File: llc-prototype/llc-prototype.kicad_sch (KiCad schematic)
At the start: 37 parts, among them J1 +HV, J2 -HV, J3 +LV, J4 -LV, Q1 MCTL011N20YH-TP, Q2 MCTL011N20YH-TP, Q3 NTMFS1D3N04XMT1G, Q4 NTMFS1D3N04XMT1G, T1 Transformer_SP_2S, U3 PC817, U4 TL431DBZ

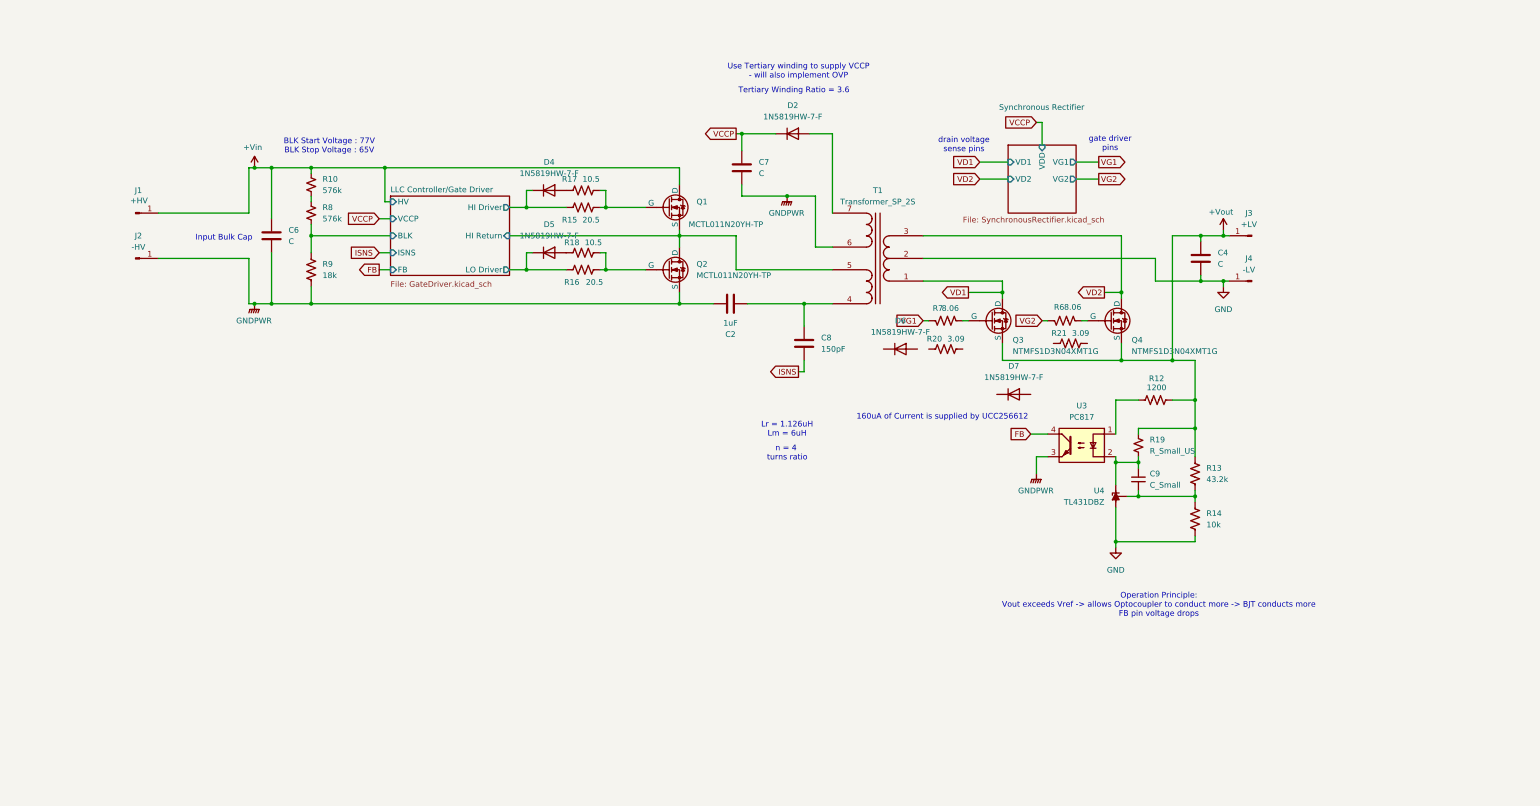
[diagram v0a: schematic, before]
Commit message: added fuses
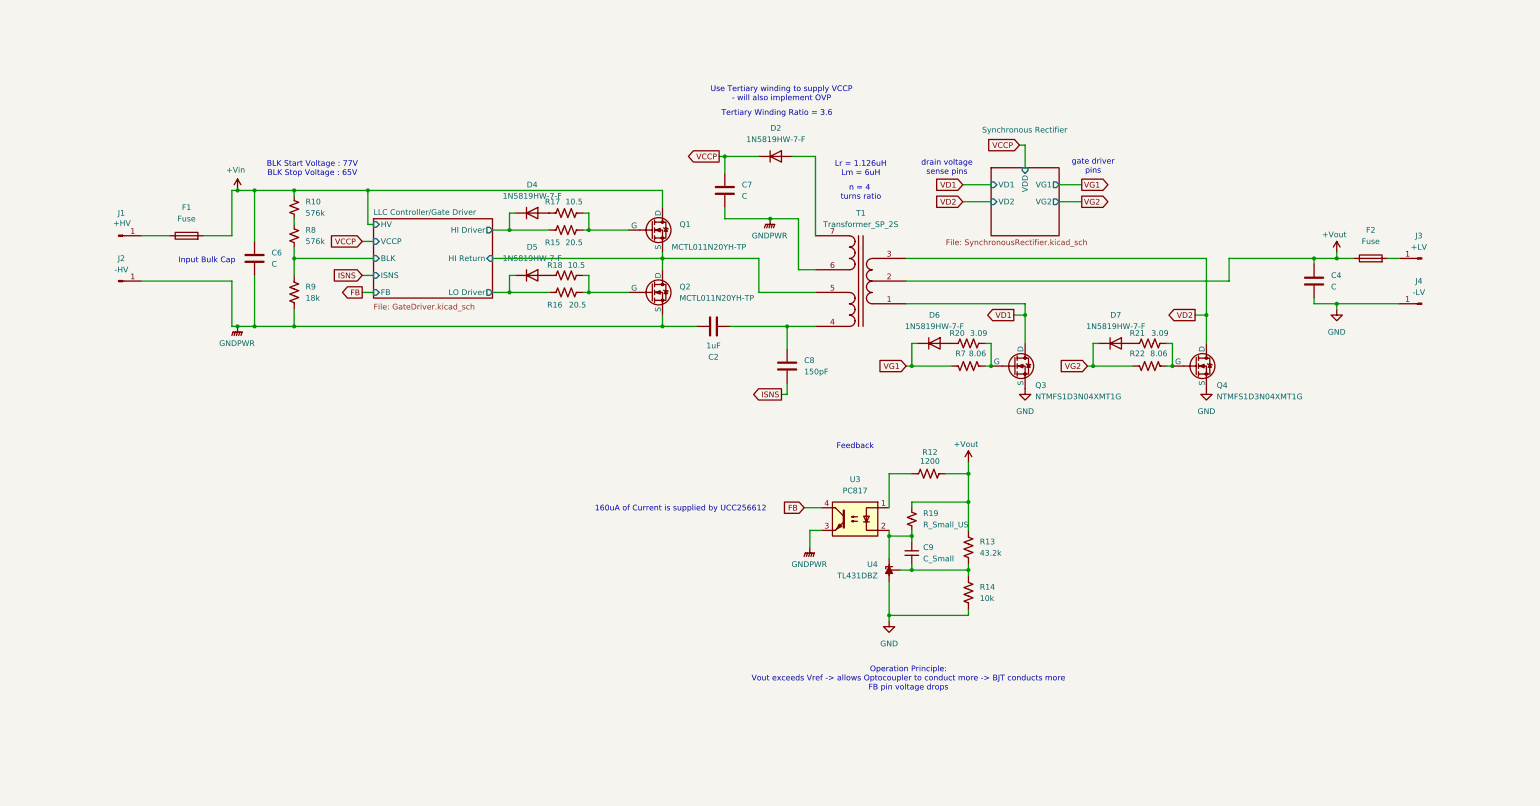
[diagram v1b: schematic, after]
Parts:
- removed R6: 8.06, Resistor_SMD:R_0603_1608Metric_Pad0.98x0.95mm_HandSolder, symbol Device:R_US
- added F1, F2: Fuse, symbol Device:Fuse
- added R22: 8.06, Resistor_SMD:R_0603_1608Metric_Pad0.98x0.95mm_HandSolder, symbol Device:R_US
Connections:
- net +Vin: now also F1.2; no longer J1.1 (Pin_1)
- net +Vout: now also T1.2 (PM), F2.1; no longer J3.1 (Pin_1), Q3.1 (S), Q4.1 (S)
- net GND: now also Q3.1 (S), Q4.1 (S); no longer T1.2 (PM)
- net VG1: now also D6.1 (K)
- net VG2: now also D7.1 (K), R22.1
- net at Q3.4 (G), R7.2: now also R20.2
- net at D7.2 (A): now also R21.1
- net at Q4.4 (G): now also R21.2, R22.2
- net at R20.1: now also D6.2 (A)
- new net: F1.1, J1.1 (Pin_1)
- new net: F2.2, J3.1 (Pin_1)
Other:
- note added: "Feedback"
- moved on the sheet: C2, C4, C6, C7, C8, C9, D2, D4, D5, D6, J1, J2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

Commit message: PCB work, added more caps
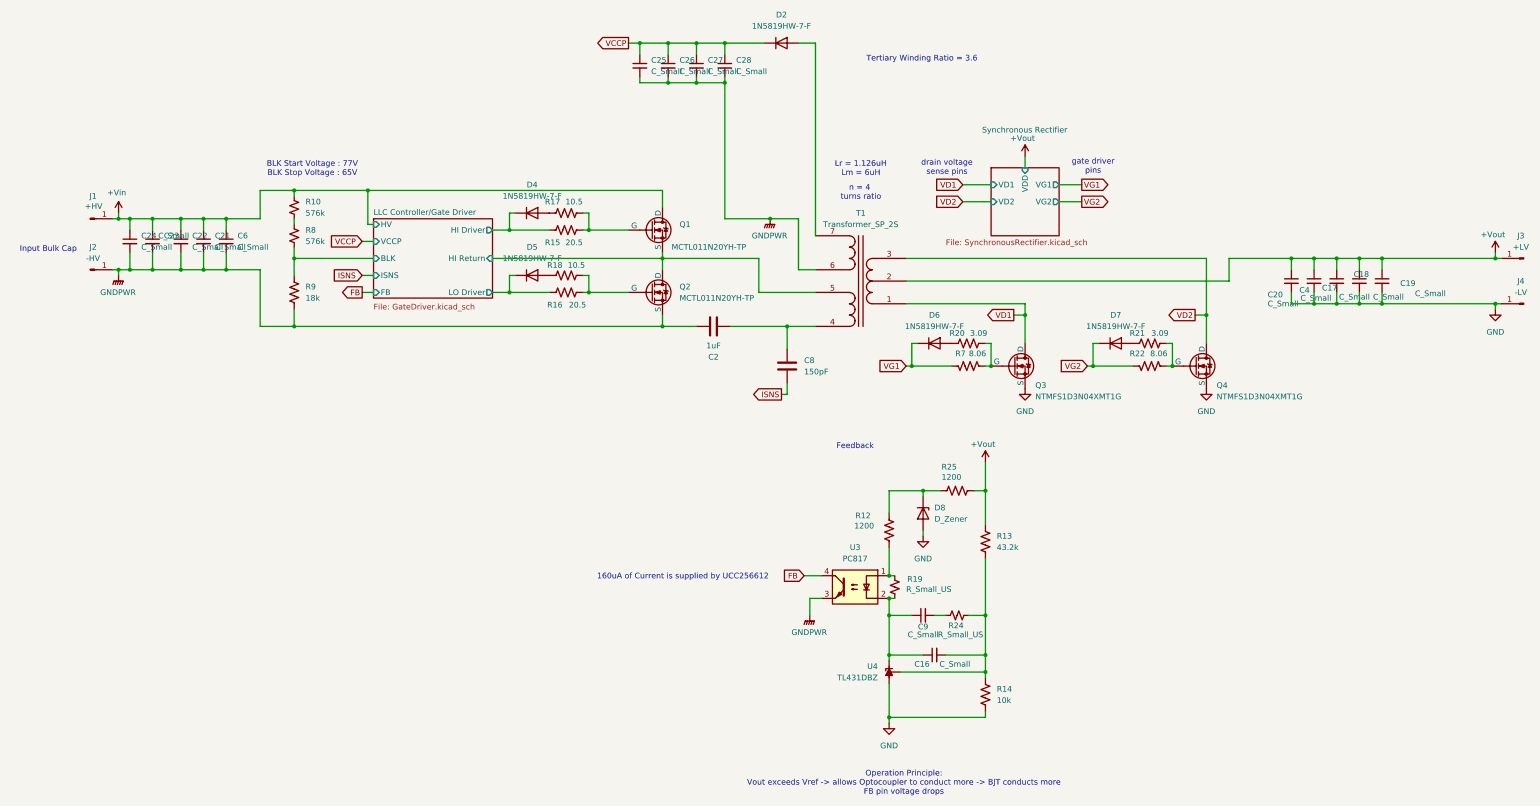
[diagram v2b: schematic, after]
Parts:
- removed C4, C6, C7: C, Capacitor_SMD:C_0603_1608Metric_Pad1.08x0.95mm_HandSolder, symbol Device:C
- removed F1, F2: Fuse, symbol Device:Fuse
- added C16, C17, C18, C19, C20, C21, C22, C23, C24, C25, C26, C27, C28, C4, C6: C_Small, Capacitor_SMD:C_0603_1608Metric_Pad1.08x0.95mm_HandSolder, symbol Device:C_Small
- added D8: D_Zener, symbol Device:D_Zener
- added R24: R_Small_US, Resistor_SMD:R_0603_1608Metric_Pad0.98x0.95mm_HandSolder, symbol Device:R_Small_US
- added R25: 1200, Resistor_SMD:R_0603_1608Metric_Pad0.98x0.95mm_HandSolder, symbol Device:R_US
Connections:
- net +Vin: now also J1.1 (Pin_1), C21.1, C22.1, C23.1, C24.1, C6.1
- net +Vout: now also J3.1 (Pin_1), C17.1, C18.1, C19.1, C20.1, C4.1, R25.2; no longer R12.1, R19.1
- net GND: now also C17.2, C18.2, C19.2, C20.2, C4.2, D8.2 (A)
- net GNDPWR: now also C21.2, C22.2, C23.2, C24.2, C25.2, C26.2, C27.2, C28.2, C6.2
- net VCCP: now also C25.1, C26.1, C27.1, C28.1
- net at R13.2, R14.1, U4.2 (REF): now also C16.2, R24.2; no longer C9.2
- net at R12.2, U3.1: now also R19.1
- net at C9.1, R19.2, U3.2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: now also C16.1
- new net: C9.2, R24.1
- new net: D8.1 (K), R12.1, R25.1
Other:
- note removed: "Use Tertiary winding to supply VCCP - will also implement OVP"
- moved on the sheet: D2, J1, J2, J3, J4, R12, R13, R14, U3, U4

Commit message: pcb changes + fs-components update
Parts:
- Q3, Q4: footprint Package_SO:ONSemi_SO-8FL_488AA -> formula_slug_footprint_library:ONSemi_SO-8FL_488AA_editedForLLC
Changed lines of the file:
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@@
 	)
 	(junction
-		(at 298.45 139.7)
-		(diameter 0)
-		(color 0 0 0 0)
-	)
-	(junction
 		(at 76.2 118.11)
 		(diameter 0)
@@
 	)
 	(junction
+		(at 298.45 139.7)
+		(diameter 0)
+		(color 0 0 0 0)
+	)
+	(junction
 		(at 184.15 115.57)
 		(diameter 0)
@@
 	)
 	(symbol
-		(lib_name "NMOS_3")
-		(lib_id "Simulation_SPICE:NMOS")
-		(at 303.53 139.7 0)
-		(unit 1)
-		(body_style 1)
-		(exclude_from_sim no)
-		(in_bom yes)
-		(on_board yes)
-		(in_pos_files yes)
-		(dnp no)
-		(property "Reference" "Q4"
-			(at 308.356 144.018 0)
-			(show_name no)
-			(do_not_autoplace no)
-			(effects
-				(font
-					(size 1.27 1.27)
-				)
-				(justify left)
-			)
-		)
-		(property "Value" "NTMFS1D3N04XMT1G"
-			(at 308.356 146.558 0)
-			(show_name no)
-			(do_not_autoplace no)
-			(effects
-				(font
-					(size 1.27 1.27)
-				)
-				(justify left)
-			)
-		)
-		(property "Footprint" "Package_SO:ONSemi_SO-8FL_488AA"
-			(at 308.61 137.16 0)
-			(hide yes)
-			(show_name no)
-			(do_not_autoplace no)
-			(effects
-				(font
-					(size 1.27 1.27)
-				)
-			)
-		)
-		(property "Datasheet" "https://www.onsemi.com/download/data-sheet/pdf/ntmfs1d3n04xm-d.pdf"
-			(at 303.53 152.4 0)
-			(hide yes)
-			(show_name no)
-			(do_not_autoplace no)
-			(effects
-				(font
-					(size 1.27 1.27)
-				)
-			)
-		)
-		(property "Description" "N-MOSFET transistor, drain/source/gate"
-			(at 303.53 139.7 0)
-			(hide yes)
-			(show_name no)
-			(do_not_autoplace no)
-			(effects
-				(font
-					(size 1.27 1.27)
-				)
-			)
-		)
-		(property "Sim.Device" "NMOS"
-			(at 303.53 156.845 0)
-			(hide yes)
-			(show_name no)
-			(do_not_autoplace no)
-			(effects
-				(font
-					(size 1.27 1.27)
-				)
-			)
-		)
-		(property "Sim.Type" "VDMOS"
-			(at 303.53 158.75 0)
-			(hide yes)
-			(show_name no)
-			(do_not_autoplace no)
-			(effects
-				(font
-					(size 1.27 1.27)
-				)
-			)
-		)
-		(property "Sim.Pins" "1=D 2=G 3=S"
-			(at 303.53 154.94 0)
-			(hide yes)
-			(show_name no)
-			(do_not_autoplace no)
-			(effects
-				(font
-					(size 1.27 1.27)
-				)
-			)
-		)
-		(property "Digikey Part Number" ""
-			(at 303.53 139.7 0)
-			(hide yes)
-			(show_name no)
-			(do_not_autoplace no)
-			(effects
-				(font
-					(size 1.27 1.27)
-				)
-			)
-		)
-		(property "Digikey URL" ""
-			(at 303.53 139.7 0)
-			(hide yes)
-			(show_name no)
-			(do_not_autoplace no)
-			(effects
-				(font
-					(size 1.27 1.27)
-				)
-			)
-		)
-		(property "Manufacturer" ""
-			(at 303.53 139.7 0)
-			(hide yes)
-			(show_name no)
-			(do_not_autoplace no)
-			(effects
-				(font
-					(size 1.27 1.27)
-				)
-			)
-		)
-		(property "Manufacturer Part Number" ""
-			(at 303.53 139.7 0)
-			(hide yes)
-			(show_name no)
-			(do_not_autoplace no)
-			(effects
-				(font
-					(size 1.27 1.27)
-				)
-			)
-		)
-		(pin "5"
-		)
-		(pin "1"
-		)
-		(pin "4"
-		)
-		(instances
-			(project "llc-prototype"
-				(path "/e994741c-7c7d-4124-9d00-43b883baa61d"
-					(reference "Q4")
-					(unit 1)
-				)
-			)
-		)
-	)
-	(symbol
 		(lib_id "Device:C_Small")
 		(at 242.57 195.58 90)
@@
 			)
 		)
-		(property "Footprint" "Package_SO:ONSemi_SO-8FL_488AA"
+		(property "Footprint" "formula_slug_footprint_library:ONSemi_SO-8FL_488AA_editedForLLC"
 			(at 267.97 137.16 0)
 			(hide yes)
@@
 					(unit 1)
 				)
+			)
+		)
+	)
+	(symbol
+		(lib_name "NMOS_2")
+		(lib_id "Simulation_SPICE:NMOS")
+		(at 303.53 139.7 0)
+		(unit 1)
+		(body_style 1)
+		(exclude_from_sim no)
+		(in_bom yes)
+		(on_board yes)
+		(in_pos_files yes)
+		(dnp no)
+		(property "Reference" "Q4"
+			(at 308.356 144.018 0)
+			(show_name no)
+			(do_not_autoplace no)
+			(effects
+				(font
+					(size 1.27 1.27)
+				)
+				(justify left)
+			)
+		)
+		(property "Value" "NTMFS1D3N04XMT1G"
+			(at 308.356 146.558 0)
+			(show_name no)
+			(do_not_autoplace no)
+			(effects
+				(font
+					(size 1.27 1.27)
+				)
+				(justify left)
+			)
+		)
+		(property "Footprint" "formula_slug_footprint_library:ONSemi_SO-8FL_488AA_editedForLLC"
+			(at 308.61 137.16 0)
+			(hide yes)
+			(show_name no)
+			(do_not_autoplace no)
+			(effects
+				(font
+					(size 1.27 1.27)
+				)
+			)
+		)
+		(property "Datasheet" "https://www.onsemi.com/download/data-sheet/pdf/ntmfs1d3n04xm-d.pdf"
+			(at 303.53 152.4 0)
+			(hide yes)
+			(show_name no)
+			(do_not_autoplace no)
+			(effects
+				(font
+					(size 1.27 1.27)
+				)
+			)
+		)
+		(property "Description" "N-MOSFET transistor, drain/source/gate"
+			(at 303.53 139.7 0)
+			(hide yes)
+			(show_name no)
+			(do_not_autoplace no)
+			(effects
+				(font
+					(size 1.27 1.27)
+				)
+			)
+		)
+		(property "Sim.Device" "NMOS"
+			(at 303.53 156.845 0)
+			(hide yes)
+			(show_name no)
+			(do_not_autoplace no)
+			(effects
+				(font
+					(size 1.27 1.27)
+				)
+			)
+		)
+		(property "Sim.Type" "VDMOS"
+			(at 303.53 158.75 0)
+			(hide yes)
+			(show_name no)
+			(do_not_autoplace no)
+			(effects
+				(font
+					(size 1.27 1.27)
+				)
+			)
+		)
+		(property "Sim.Pins" "1=D 2=G 3=S"
+			(at 303.53 154.94 0)
+			(hide yes)
+			(show_name no)
+			(do_not_autoplace no)
+			(effects
+				(font
+					(size 1.27 1.27)
+				)
+			)
+		)
+		(property "Digikey Part Number" ""
+			(at 303.53 139.7 0)
+			(hide yes)
+			(show_name no)
+			(do_not_autoplace no)
+			(effects
+				(font
+					(size 1.27 1.27)
+				)
+			)
+		)
+		(property "Digikey URL" ""
+			(at 303.53 139.7 0)
+			(hide yes)
+			(show_name no)
+			(do_not_autoplace no)
+			(effects
+				(font
+					(size 1.27 1.27)
+				)
+			)
+		)
+		(property "Manufacturer" ""
+			(at 303.53 139.7 0)
+			(hide yes)
+			(show_name no)
+			(do_not_autoplace no)
+			(effects
+				(font
+					(size 1.27 1.27)
+				)
+			)
+		)
+		(property "Manufacturer Part Number" ""
+			(at 303.53 139.7 0)
+			(hide yes)
+			(show_name no)
+			(do_not_autoplace no)
+			(effects
+				(font
+					(size 1.27 1.27)
+				)
+			)
+		)
+		(pin "5"
+		)
+		(pin "1"
+		)
+		(pin "4"
+		)
+		(instances
+			(project "llc-prototype"
+				(path "/e994741c-7c7d-4124-9d00-43b883baa61d"
+					(reference "Q4")
+					(unit 1)
+				)

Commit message: changed hb mosfet footprint
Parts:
- Q1, Q2: footprint Package_TO_SOT_SMD:Infineon_PG-HSOF-8-1_ThermalVias -> Package_TO_SOT_SMD:Infineon_PG-HSOF-8-1
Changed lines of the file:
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@@
 			)
 		)
-		(property "Footprint" "Package_TO_SOT_SMD:Infineon_PG-HSOF-8-1_ThermalVias"
+		(property "Footprint" "Package_TO_SOT_SMD:Infineon_PG-HSOF-8-1"
 			(at 186.69 120.65 0)
 			(hide yes)
@@
 			)
 		)
-		(property "Footprint" "Package_TO_SOT_SMD:Infineon_PG-HSOF-8-1_ThermalVias"
+		(property "Footprint" "Package_TO_SOT_SMD:Infineon_PG-HSOF-8-1"
 			(at 186.69 106.68 0)
 			(hide yes)
